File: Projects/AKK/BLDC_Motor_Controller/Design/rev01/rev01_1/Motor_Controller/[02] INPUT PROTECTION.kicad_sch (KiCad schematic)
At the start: 0 parts

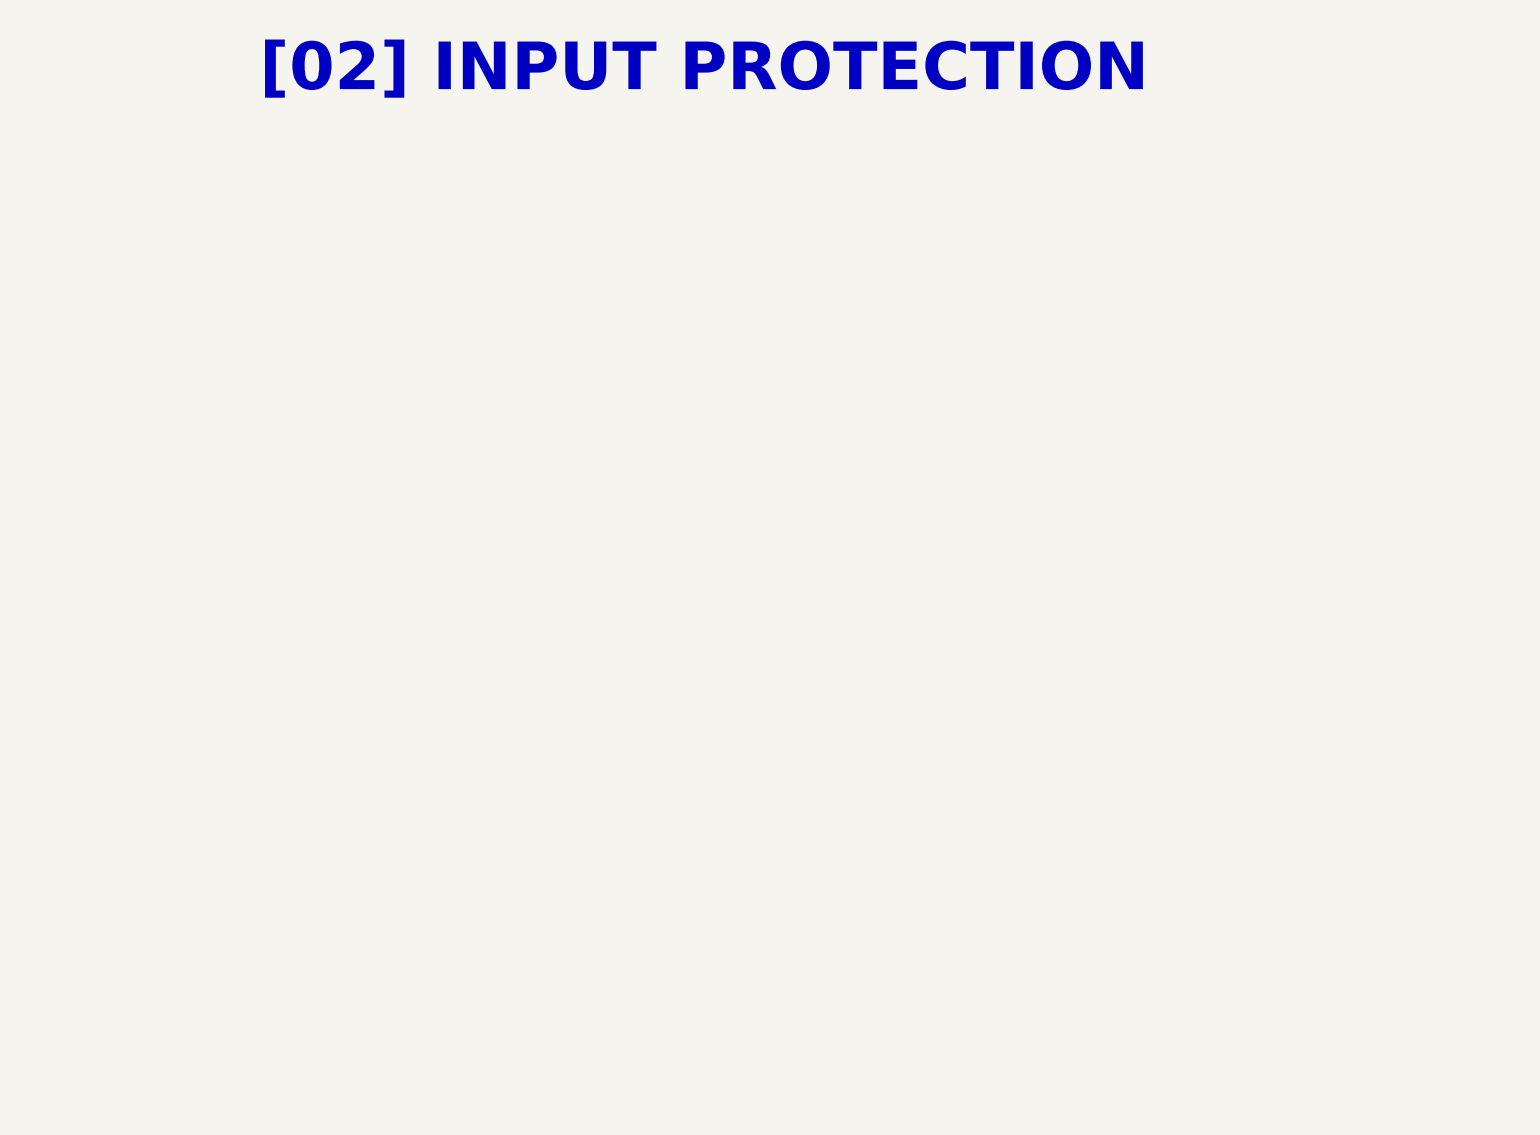
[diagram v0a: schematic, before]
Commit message: Update_03
Completed schematic.
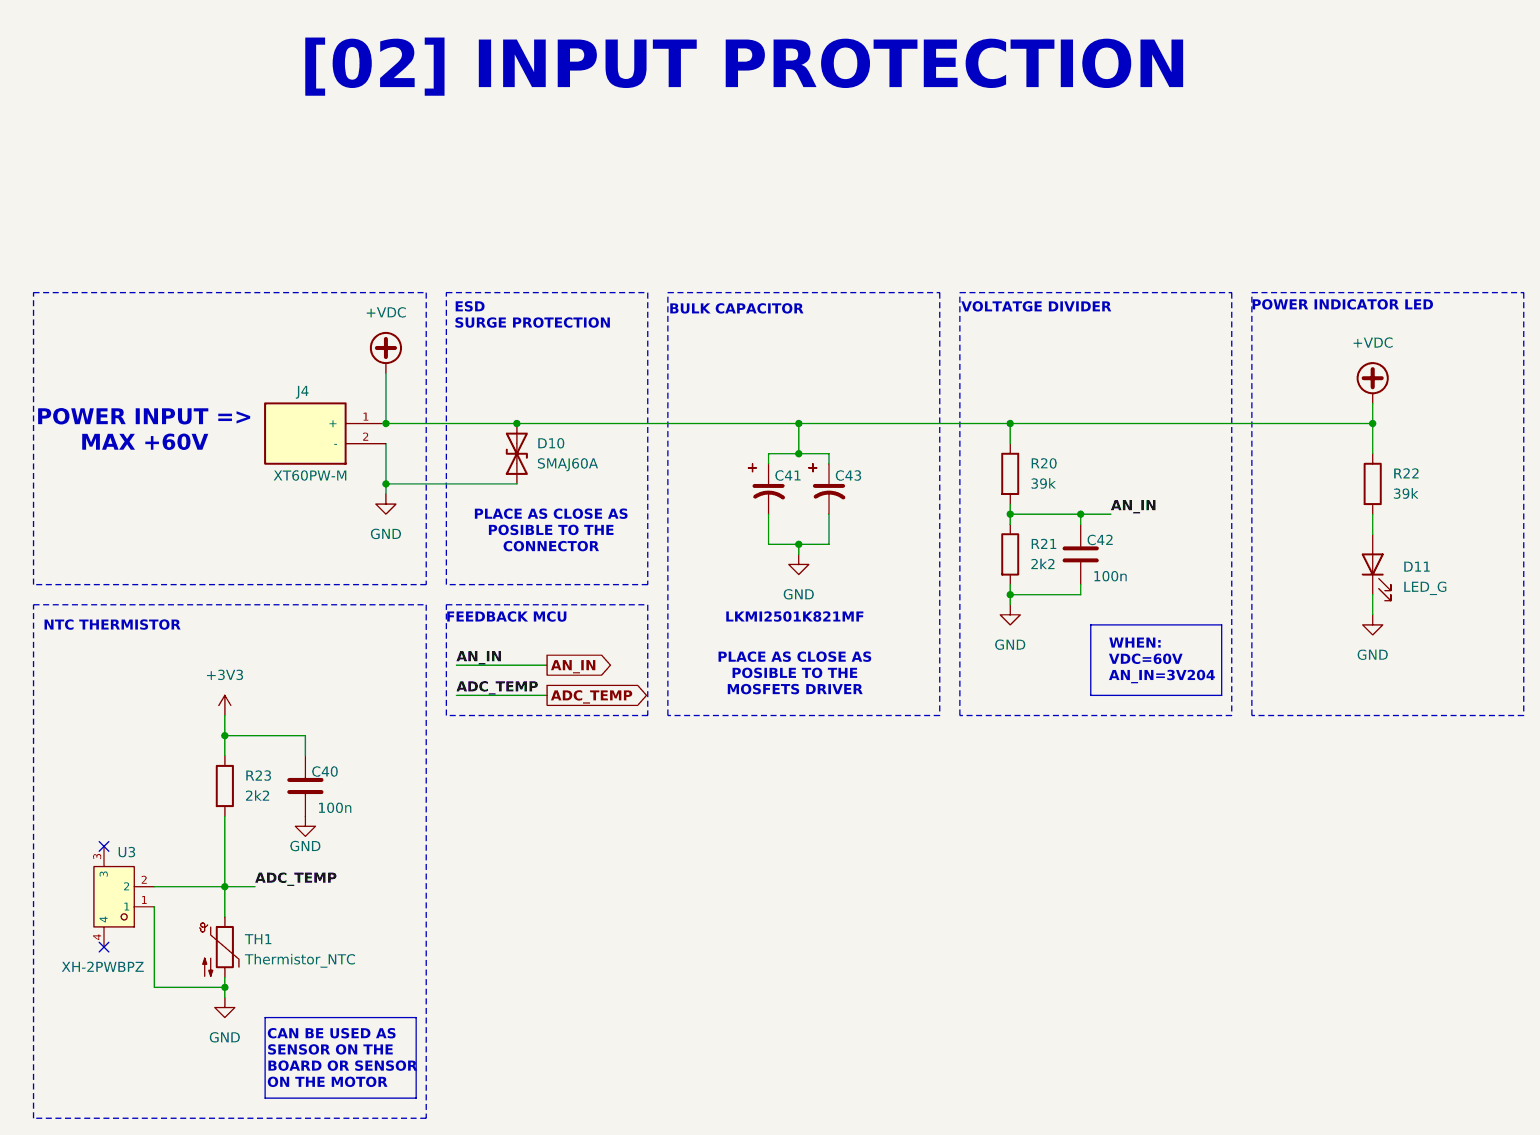
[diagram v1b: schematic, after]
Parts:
- added C40, C42: 100n, symbol Device:C
- added C41, C43: LKMI2501K821MF, LKMI2501K821MF_footprint_lib:CAP-TH_BD16.0-P7.50-D1.2-FD, symbol LKMI2501K821MF:LKMI2501K821MF
- added D10: SMAJ60A, symbol Device:D_TVS
- added D11: LED_G, symbol Device:LED
- added J4: XT60PW-M, XT60PW-M:AMASS_XT60PW-M, symbol XT60PW:XT60PW-M
- added R20, R22: 39k, symbol Device:R
- added R21, R23: 2k2, symbol Device:R
- added TH1: Thermistor_NTC, symbol Device:Thermistor_NTC
- added U3: XH-2PWBPZ, CONN_footprint_lib:CONN-SMD_XH-2PWBPZ, symbol XH-2PWBPZ:XH-2PWBPZ
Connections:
- new net: D11.2 (A), R22.2
- new net +3V3: C40.1, R23.1
- new net +VDC: C41.1, C43.1, D10.2 (A2), J4.1 (+), R20.1, R22.1
- new net ADC_TEMP: R23.2, TH1.1, U3.2
- new net AN_IN: C42.1, R20.2, R21.1
- new net GND: C40.2, C41.2, C42.2, C43.2, D10.1 (A1), D11.1 (K), J4.2 (-), R21.2, TH1.2, U3.1
- no-connect marks 0 -> 2
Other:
- note added: "BULK CAPACITOR"
- note added: "CAN BE USED AS SENSOR ON THE BOARD OR SENSOR ON THE MOTOR"
- note added: "ESD SURGE PROTECTION"
- note added: "FEEDBACK MCU"
- note added: "LKMI2501K821MF"
- note added: "NTC THERMISTOR"
- note added: "PLACE AS CLOSE AS POSIBLE TO THE CONNECTOR"
- note added: "PLACE AS CLOSE AS POSIBLE TO THE MOSFETS DRIVER"
- note added: "POWER INDICATOR LED"
- note added: "POWER INPUT => MAX +60V"
- note added: "VOLTATGE DIVIDER"
- note added: "WHEN: VDC=60V AN_IN=3V204"
